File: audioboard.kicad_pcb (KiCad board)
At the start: 4 copper layers, 34 x 34 mm, 72 parts, among them IC1 TP4054-42-SOT25-R, J1 GCT_USB4125, J2 Conn_01x02, J3 Audio, J4 SJ-43514-SMT, J5 JTAG, J6 UART, J7 GPIO, Q1 AO3401A, SW1 RESET, U1 ES8388, U2 ESP32-PICO-D4, U3 AMS1117-3.3

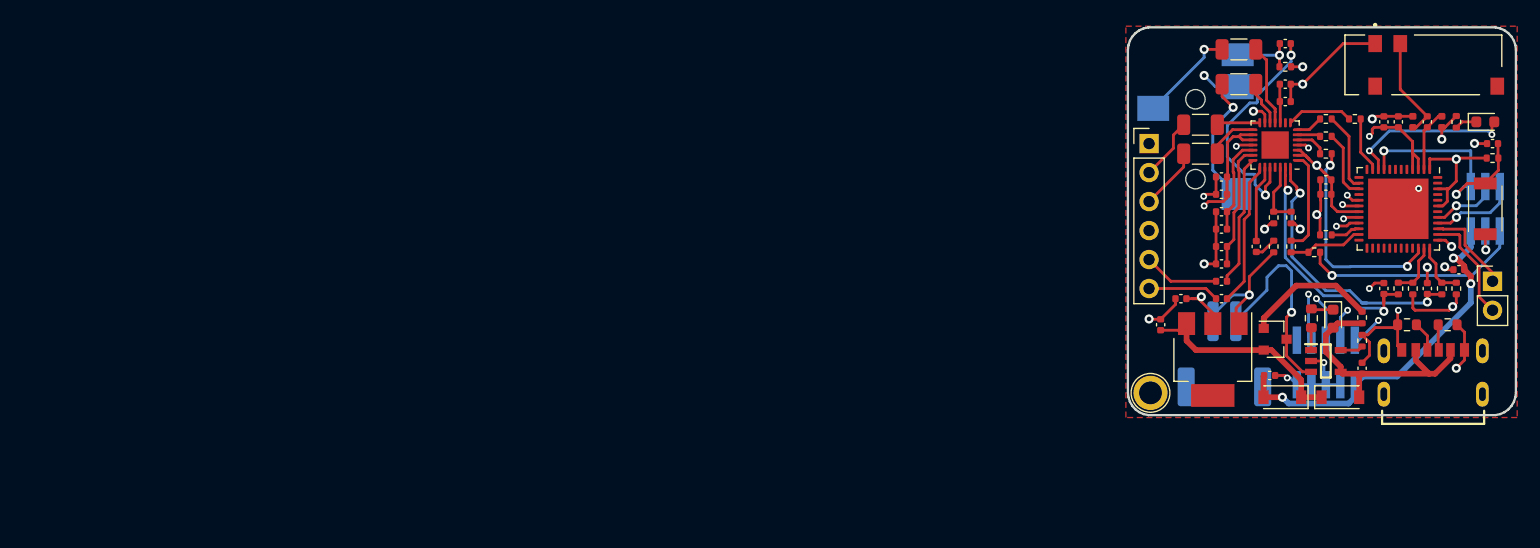
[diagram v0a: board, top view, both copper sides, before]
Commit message: Add v2
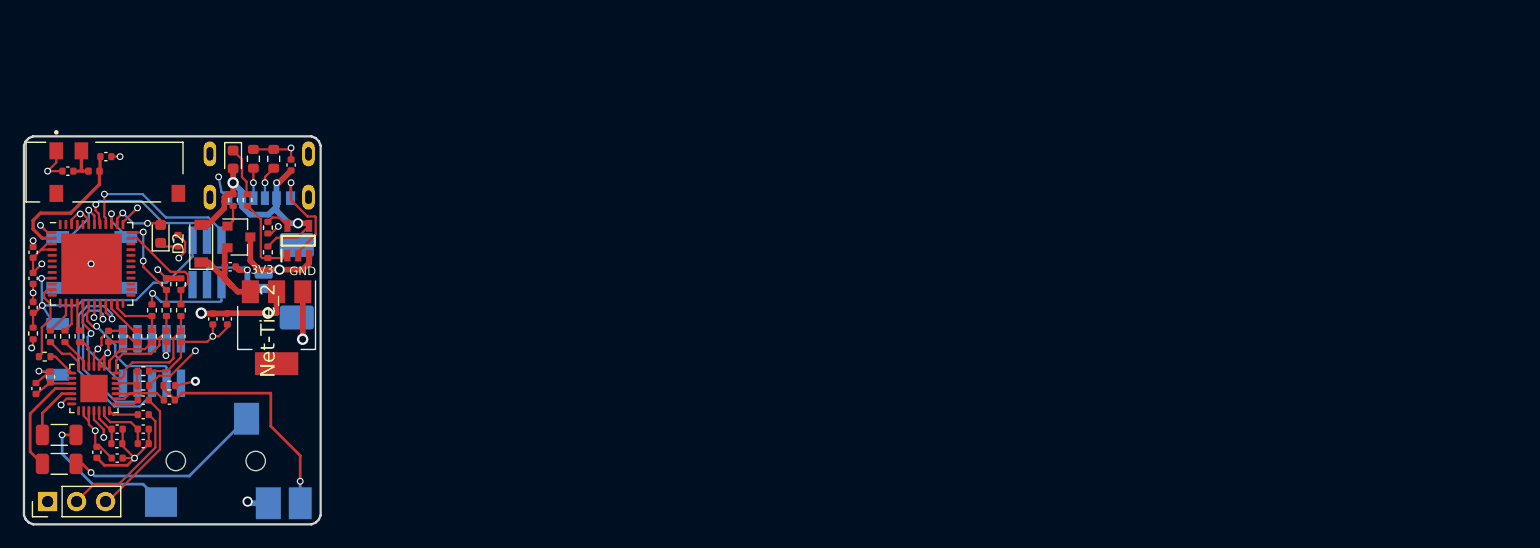
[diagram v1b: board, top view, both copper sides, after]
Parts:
- removed C23: 1uF, Capacitor_SMD:C_0402_1005Metric
- removed C30, C31: 47uF, Capacitor_SMD:C_1206_3216Metric
- removed C33, C34: 100nF, Capacitor_SMD:C_0402_1005Metric
- removed D3: B5819, Diode_SMD:D_SOD-123
- removed J7: GPIO, Connector_PinHeader_2.54mm:PinHeader_1x02_P2.54mm_Vertical
- removed L2: 4.7nH, Inductor_SMD:L_0402_1005Metric
- removed REF**: TestPoint_Plated_Hole_D2.0mm, TestPoint:TestPoint_Plated_Hole_D2.0mm
- added C14: 2.2nF, Capacitor_SMD:C_0402_1005Metric, F.Cu at (80.3, 79.2)
- added C3: 10uF, Capacitor_SMD:C_0402_1005Metric, F.Cu at (94.2, 92.2)
- added NT1: Net-Tie_2, NetTie:NetTie-2_SMD_Pad0.5mm, F.Cu at (99.3, 94.0)
- added NT2: Net-Tie_2, NetTie:NetTie-2_SMD_Pad0.5mm, B.Cu at (97.8, 93.2)
- added SW2: RESET, audioboard:TS1088R02026, B.Cu at (79.4, 87.2)
- added SW3: RESET, audioboard:TS1088R02026, B.Cu at (85.3, 87.2)
- C2: value 1pF -> 4.7nF
- J1, SW1: moved to B.Cu
- J2: footprint Connector_JST:JST_PH_S2B-PH-SM4-TB_1x02-1MP_P2.00mm_Horizontal -> Connector_Molex:Molex_PicoBlade_53261-0271_1x02-1MP_P1.25mm_Horizontal
- J3: footprint Connector_PinHeader_2.54mm:PinHeader_1x06_P2.54mm_Vertical -> Connector_PinHeader_2.54mm:PinHeader_1x03_P2.54mm_Vertical
- L1: value 2.7nH -> 0nH
- R4: footprint Resistor_SMD:R_0603_1608Metric -> Resistor_SMD:R_0402_1005Metric
- R5: value 10k -> 3.3k
- moved R1 128.8 mm to (77.2, 93.5), turned to 270 degrees
- moved C1 128.7 mm to (77.2, 91.2), turned to 90 degrees
- moved SW1 125.7 mm to (79.4, 94.9)
- moved C11 120.2 mm to (77.2, 86.4)
- moved C9 119.2 mm to (77.2, 88.6), turned to 270 degrees
- moved R11 116.7 mm to (78.2, 95.5), turned to 180 degrees
- moved D4 116.5 mm to (88.4, 84.7), turned to 90 degrees
- moved E1 116.0 mm to (79.2, 77.5)
- moved C2 115.8 mm to (83.6, 78.0), turned to 180 degrees
- moved L1 115.7 mm to (82.5, 79.2), turned to 0 degrees
- moved U2 114.6 mm to (82.3, 87.4), turned to 0 degrees
- moved R9 113.4 mm to (78.7, 93.7), turned to 90 degrees
- moved R18 113.0 mm to (88.9, 89.2), turned to 90 degrees
- moved R22 112.5 mm to (89.9, 85.3)
- moved C15 112.3 mm to (77.5, 98.3), turned to 90 degrees
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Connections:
- C16 pad 1: GND -> ADCVREF
- C16 pad 2: ADCVREF -> GNDA
- C17 pad 2: GND -> GNDA
- C18 pad 1: +3V3 -> +3.3VA
- C18 pad 2: GND -> GNDA
- C2 pad 1: Net-(C2-Pad1) -> GND
- C20 pad 1: +3V3 -> +3.3VA
- C20 pad 2: GND -> GNDA
- C7 pad 1: GND -> ADCVREF
- C7 pad 2: ADCVREF -> GNDA
- C8 pad 2: GND -> GNDA
- E1 pad 2: Net-(C2-Pad1) -> Net-(C14-Pad2)
- J3 pad 1: GND -> GNDA
- J3 pad 2: LINEOUT_R -> LINEIN_R
- J3 pad 3: LINEOUT_L -> LINEIN_L
- J4 pad 4: GND -> GNDA
- J5 pad 1: VCC -> Net-(J5-Pad1)
- J6 pad 2: VCC -> Net-(J6-Pad2)
- L1 pad 1: Net-(C2-Pad1) -> Net-(C14-Pad2)
- L1 pad 2: GND -> Ant
- R16 pad 1: GND -> Net-(IC1-Pad1)
- R16 pad 2: Net-(C23-Pad1) -> VBUS
- R6 pad 2: +3V3 -> +3.3VA
- U1 pad 13: GND -> GNDA
- U1 pad 16: +3V3 -> +3.3VA
- U1 pad 17: +3V3 -> +3.3VA
- U1 pad 18: GND -> GNDA
- U1 pad 23: Net-(C23-Pad2) -> Net-(C24-Pad2)
- U2 pad 10: STATUS_LED -> Net-(U2-Pad10)
- U2 pad 16: Net-(U2-Pad16) -> I2S_BCLK
- U2 pad 34: I2S_BCLK -> Net-(U2-Pad34)
- U2 pad 38: GPIO19 -> STATUS_LED
- U2 pad 39: GPIO22 -> IO22
- U2 pad 42: Net-(U2-Pad42) -> IO21
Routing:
- net GNDA: track 0.00 -> 33.8 mm, vias 0 -> 4
- net VCC: track 33.7 -> 0.00 mm, vias 3 -> 0
- net +3.3VA: track 0.00 -> 26.7 mm, vias 0 -> 2
- net +3V3: track 57.3 -> 37.9 mm, vias 9 -> 11
- net I2S_BCLK: track 19.2 -> 2.47 mm, vias 2 -> 0
- net Net-(C27-Pad1): track 24.5 -> 8.30 mm, vias 2 -> 0
- net HP_MIC: track 5.73 -> 21.1 mm
- net GND: track 90.7 -> 75.9 mm, vias 23 -> 16
- net Net-(C24-Pad2): track 20.4 -> 6.61 mm, vias 2 -> 0
- net Net-(C22-Pad1): track 22.3 -> 9.96 mm, vias 2 -> 0
- net IO0: track 19.7 -> 8.78 mm
- net Net-(C26-Pad2): track 12.7 -> 2.03 mm
- net GPIO19: track 9.71 -> 0.00 mm
- net STATUS_LED: track 14.7 -> 5.04 mm
- net Net-(Q1-Pad1): track 11.6 -> 1.97 mm
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- added copper zone on In1.Cu, net GNDA
- removed copper zone on F.Cu, net GND
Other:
- board size 34 x 34 mm -> 26 x 34 mm
- net class Default: trace_width 0.25 -> 0.2; via_dia 0.8 -> 0.6
- rule trace_min: 0.2 -> 0.09
- rule via_min_drill: 0.3 -> 0.2
- rule via_min_size: 0.45 -> 0.4
